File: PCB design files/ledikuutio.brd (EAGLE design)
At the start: 120.6 x 83.5 mm, 54 parts, among them IC1 ATMEGA328P, IC3 74HC595D, Q2 MOSFET-NCHANNELSMD, Q3 16mhz, T1 TIP42, T2 TIP42, T3 TIP42, T4 TIP42, T5 TIP42, T6 TIP42, T7 TIP42, T8 TIP42, X1 2516-, X2 5566-20, X3 2516-, X4 2516-, X5 2516-, X6 2510-

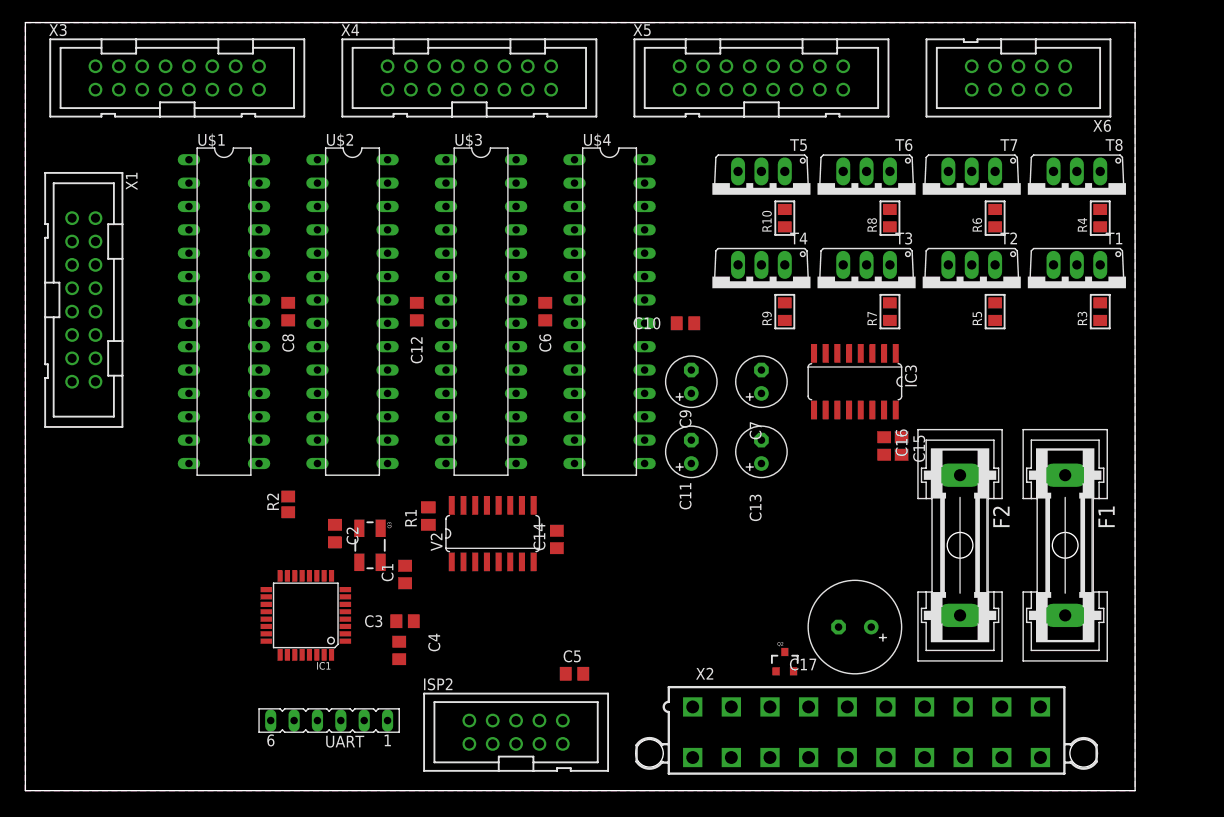
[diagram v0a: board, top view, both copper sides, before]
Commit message: Updated the designs...
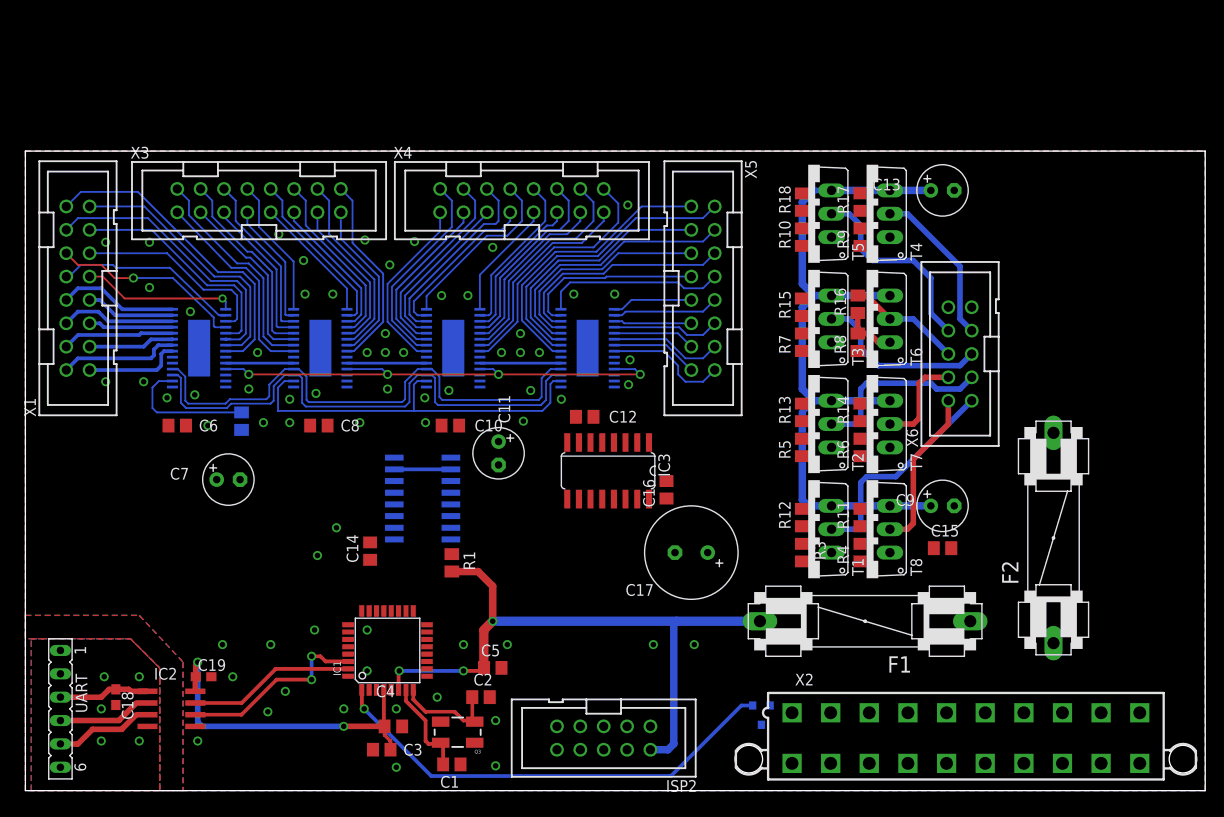
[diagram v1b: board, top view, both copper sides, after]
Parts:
- added C18, C19: 100nF, rcl:C0603
- added IC2: ISO7221A, texas:SO-08
- added R11, R12, R13, R14, R15, R16, R17, R18: 1k, rcl:M0805
- F1, F2: value (none) -> 2A; device fuse:GSH15 -> special:FUSE
- R10, R3, R4, R5, R6, R7, R8, R9: device rc-master:R0805 -> rcl:M0805
- R2: device resistor:R0805 -> rcl:M0805
- U$1, U$2, U$3, U$4: value TLC5940TLC5940NT -> TLC5940TLC5940PWP; device elovalo:DIL28 -> elovalo:PWP28
- moved C7 58.9 mm to (22.1, 33.8), turned to 0 degrees
- moved R4 44.7 mm to (90.8, 25.9)
- moved T8 42.9 mm to (91.4, 28.4), turned to 90 degrees
- moved C6 41.9 mm to (16.5, 39.7), turned to 0 degrees
- moved R3 41.7 mm to (84.5, 25.9), turned to 270 degrees
- moved T1 39.2 mm to (85.1, 28.4), turned to 90 degrees
- moved C13 34.6 mm to (99.7, 65.2), turned to 0 degrees
- moved X6 30.7 mm to (101.6, 47.5), turned to 90 degrees
- moved C9 30.5 mm to (99.7, 31.0), turned to 0 degrees
- moved UART 29.2 mm to (3.81, 8.89), turned to 270 degrees
- moved R6 28.9 mm to (90.8, 37.3)
- moved IC3 28.5 mm to (63.3, 34.8)
- moved C10 27.9 mm to (46.2, 39.7), turned to 0 degrees
- moved T7 27.4 mm to (91.4, 39.8), turned to 90 degrees
- moved R5 25.6 mm to (84.5, 37.3)
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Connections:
- removed net DCPRG: IC1.10, U$1.19, U$2.19, U$3.19, U$4.19
- removed net VPRG: IC1.9, U$1.27, U$2.27, U$3.27, U$4.27
- new net GND1: C18.2, IC2.4, UART.1
- new net RXD_FT232R: IC2.3, UART.5
- new net TXD_FT232R: IC2.2, UART.4
- new net VDD: C18.1, IC2.1, UART.3
- net +5V: now also F2.2, IC3.10, U$1.28, U$2.28, U$3.28, U$4.28; no longer F1.1, U$1.21, U$2.21, U$3.21, U$4.21
- net BLANK: now also IC1.14, U$1.2, U$2.2, U$3.2, U$4.2; no longer IC1.11, U$1.23, U$2.23, U$3.23, U$4.23
- net GND: now also C19.2, IC2.5, U$1.1, U$1.26, U$1.6, U$1.THERMAL, U$2.1, U$2.26, U$2.6, U$2.THERMAL, U$3.1, U$3.26, U$3.6, U$3.THERMAL, U$4.1, U$4.26, U$4.6, U$4.THERMAL; no longer U$1.22, U$2.22, U$3.22, U$4.22, UART.1
- net GSCLK/4: now also U$1.25, U$2.25, U$3.25, U$4.25; no longer U$1.18, U$2.18, U$3.18, U$4.18
- net MOSI: now also U$1.5; no longer U$1.26
- net N$1: now also U$1.24, U$2.5; no longer U$1.17, U$2.26
- net N$10: now also R18.2
- net N$11: now also R12.2
- net N$12: now also R13.2
- net N$13: now also R15.2
- net N$14: now also R17.2
- net N$23: now also R13.1
- net N$24: now also R12.1
- net N$25: now also R11.1
- net N$26: now also R14.1
- net N$27: now also R15.1
- net N$28: now also R16.1
- net N$29: now also R17.1
- net N$30: now also R18.1
- net N$32: now also U$1.7; no longer U$1.28
- net N$33: now also U$1.8; no longer U$1.1
- net N$34: now also U$1.9; no longer U$1.2
- net N$35: now also U$1.10; no longer U$1.3
- net N$36: now also U$1.11; no longer U$1.4
- net N$37: now also U$1.12; no longer U$1.5
- net N$38: now also U$1.13; no longer U$1.6
- net N$39: now also U$1.14; no longer U$1.7
- net N$4: now also U$2.24, U$3.5; no longer U$2.17, U$3.26
- net N$40: now also U$1.15; no longer U$1.8
- net N$41: now also U$1.16; no longer U$1.9
- net N$42: now also U$1.17; no longer U$1.10
- net N$43: now also U$1.18; no longer U$1.11
- net N$44: now also U$1.19; no longer U$1.12
- net N$45: now also U$1.20; no longer U$1.13
- net N$46: now also U$1.21; no longer U$1.14
- net N$47: now also U$1.22; no longer U$1.15
- net N$48: now also F2.1; no longer F1.2
- net N$49: now also U$2.7; no longer U$2.28
- net N$5: now also F1.1; no longer F2.2
- net N$50: now also U$2.8; no longer U$2.1
- net N$51: now also U$2.9; no longer U$2.2
- net N$52: now also U$2.10; no longer U$2.3
- net N$53: now also U$2.11; no longer U$2.4
- net N$54: now also U$2.12; no longer U$2.5
- net N$55: now also U$2.13; no longer U$2.6
- net N$56: now also U$2.14; no longer U$2.7
- net N$57: now also U$2.15; no longer U$2.8
- net N$58: now also U$2.16; no longer U$2.9
- net N$59: now also U$2.17; no longer U$2.10
- net N$60: now also U$2.18; no longer U$2.11
- net N$61: now also U$2.19; no longer U$2.12
- net N$62: now also U$2.20; no longer U$2.13
- net N$63: now also U$2.21; no longer U$2.14
- net N$64: now also U$2.22; no longer U$2.15
- net N$65: now also U$3.7; no longer U$3.28
- net N$66: now also U$3.8; no longer U$3.1
- net N$67: now also U$3.9; no longer U$3.2
- net N$68: now also U$3.10; no longer U$3.3
- net N$69: now also U$3.11; no longer U$3.4
- net N$7: now also R11.2
- net N$70: now also U$3.12; no longer U$3.5
- net N$71: now also U$3.13; no longer U$3.6
- net N$72: now also U$3.14; no longer U$3.7
- net N$73: now also U$3.15; no longer U$3.8
- net N$74: now also U$3.16; no longer U$3.9
- net N$75: now also U$3.17; no longer U$3.10
- net N$76: now also U$3.18; no longer U$3.11
- net N$77: now also U$3.19; no longer U$3.12
- net N$78: now also U$3.20; no longer U$3.13
- net N$79: now also U$3.21; no longer U$3.14
- net N$8: now also R14.2
- net N$80: now also U$3.22; no longer U$3.15
- net N$81: now also U$4.7; no longer U$4.28
- net N$82: now also U$4.8; no longer U$4.1
- net N$83: now also U$4.9; no longer U$4.2
- net N$84: now also U$4.10; no longer U$4.3
- net N$85: now also U$4.11; no longer U$4.4
- net N$86: now also U$4.12; no longer U$4.5
- net N$87: now also U$4.13; no longer U$4.6
- net N$88: now also U$4.14; no longer U$4.7
- net N$89: now also U$4.15; no longer U$4.8
- net N$9: now also R16.2
- net N$90: now also U$4.16; no longer U$4.9
- net N$91: now also U$4.17; no longer U$4.10
- net N$92: now also U$4.18; no longer U$4.11
- net N$93: now also U$4.19; no longer U$4.12
- net N$94: now also U$4.20; no longer U$4.13
- net N$95: now also U$4.21; no longer U$4.14
- net N$96: now also U$4.22; no longer U$4.15
- net N$97: now also U$3.24, U$4.5; no longer U$3.17, U$4.26
- net PS_ON: now also IC1.1; no longer IC1.2
- net RXD: now also IC2.6; no longer UART.4
- net SCLK: now also U$1.4, U$2.4, U$3.4, U$4.4; no longer U$1.25, U$2.25, U$3.25, U$4.25
- net TLC_SOUT: now also U$4.24; no longer U$4.17
- net TXD: now also IC2.7; no longer UART.5
- net VCC: now also C19.1, F1.2, IC2.8; no longer F2.1, IC3.10, UART.3
- net XLAT: now also U$1.3, U$2.3, U$3.3, U$4.3; no longer U$1.24, U$2.24, U$3.24, U$4.24
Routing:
- net VCC: track 0.00 -> 108.3 mm, vias 0 -> 5
- net +5V: track 0.00 -> 80.4 mm
- net XLAT: track 0.00 -> 58.8 mm
- net SCLK: track 0.00 -> 58.5 mm
- net BLANK: track 0.00 -> 57.0 mm
- net GSCLK/4: track 0.00 -> 55.3 mm, vias 0 -> 4
- net PS_ON: track 0.00 -> 50.6 mm, vias 0 -> 1
- net N$47: track 0.00 -> 35.0 mm
- net N$82: track 0.00 -> 32.5 mm
- net N$81: track 0.00 -> 31.4 mm
- net N$45: track 0.00 -> 30.5 mm
- net N$46: track 0.00 -> 29.5 mm
- net N$84: track 0.00 -> 28.7 mm
- net N$80: track 0.00 -> 27.6 mm
- net N$83: track 0.00 -> 27.5 mm
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- added copper zone on layer 16, net B_CUT_ISOLATION
- added copper zone on layer 1, net GND1
- added copper zone on layer 16, net GND1
- added copper zone on layer 1, net T_CUT_ISOLATION
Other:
- board size 120.6 x 83.5 mm -> 128.2 x 69.5 mm
